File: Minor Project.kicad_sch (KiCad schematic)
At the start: 32 parts, among them J1 Conn_Coaxial, J2 Conn_Coaxial, J3 Conn_Coaxial, J4 Conn_Coaxial, J5 Conn_Coaxial, J6 Conn_Coaxial, J7 Conn_Coaxial, J8 Conn_Coaxial, J9 Conn_Coaxial, U1 HMC596LP4E, U2 HMC596LP4E, U3 HMC595A, U4 DPX165850DT-8085D3, U5 HMC8410LP2FE, U6 ADL5507ACBZ

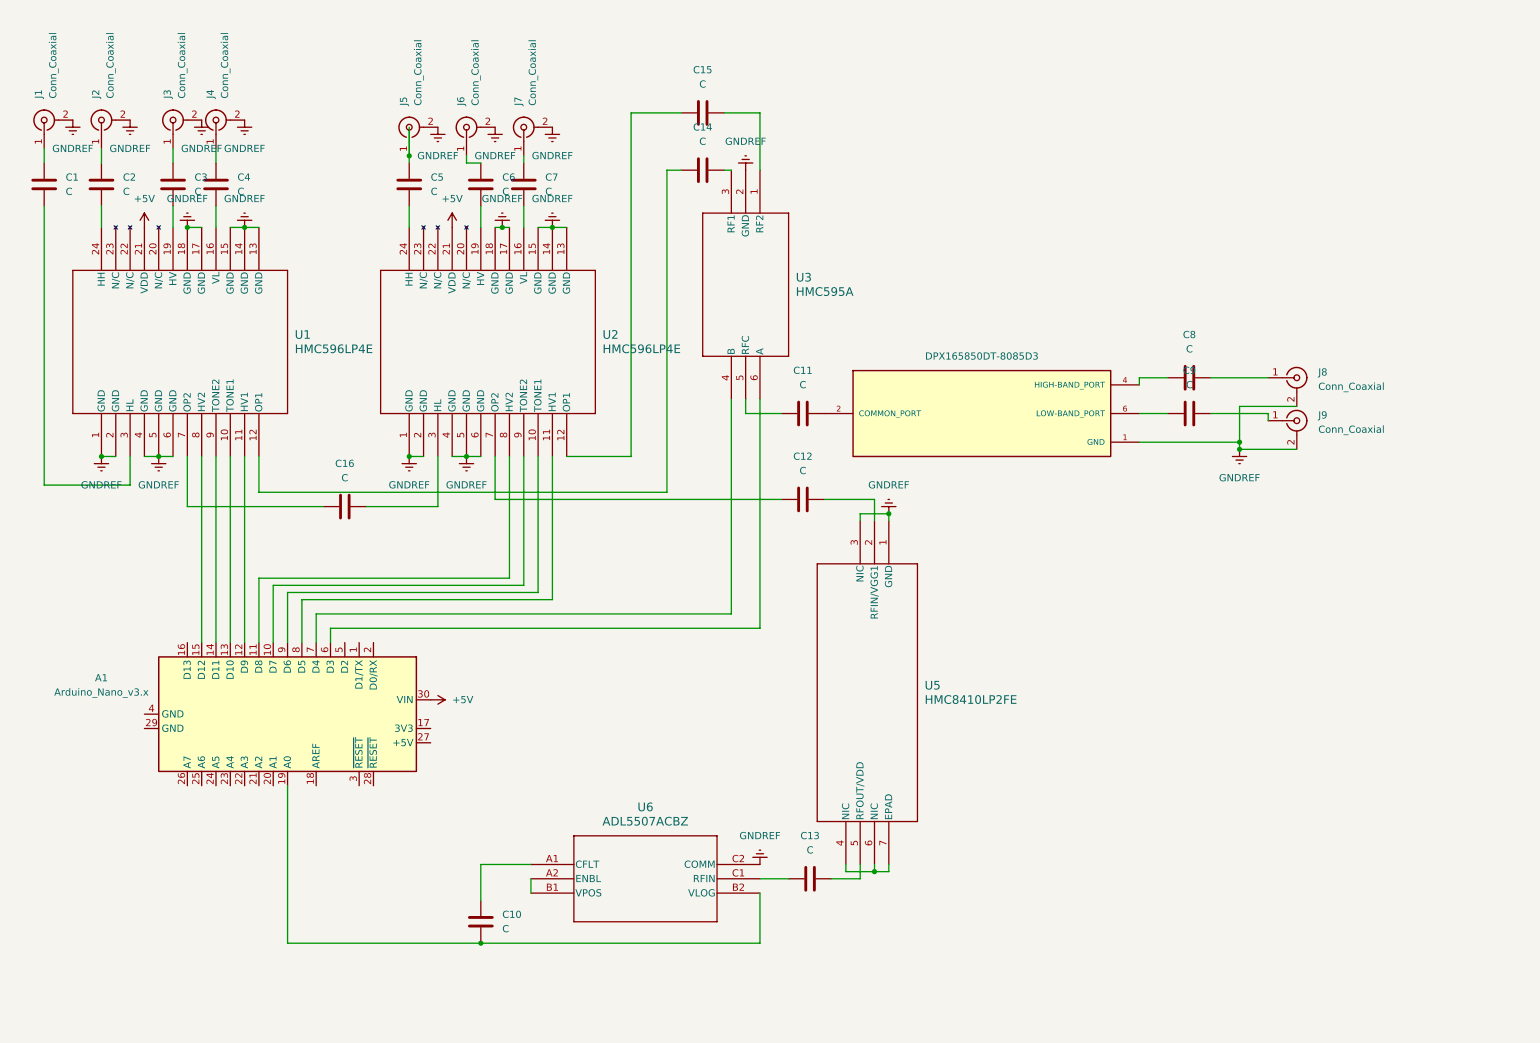
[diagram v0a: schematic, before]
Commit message: refactor schematic
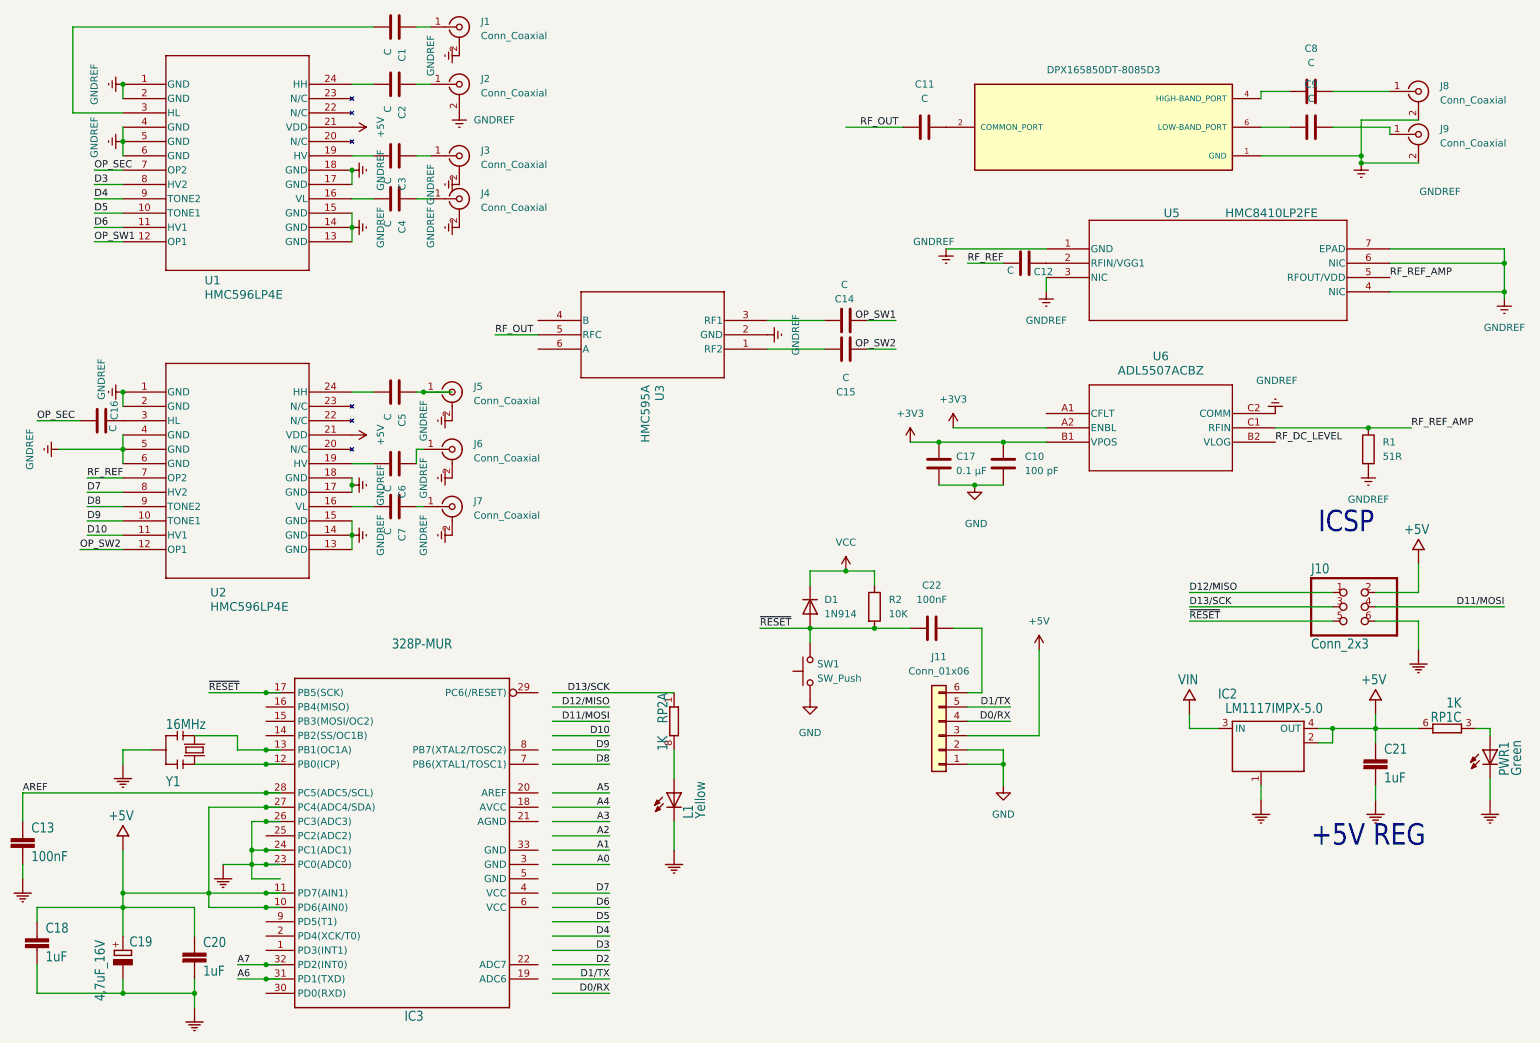
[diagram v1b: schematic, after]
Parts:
- removed A1: Arduino_Nano_v3.x, Module:Arduino_Nano, symbol MCU_Module:Arduino_Nano_v3.x
- removed C13: C, Capacitor_SMD:C_0402_1005Metric, symbol Device:C
- added C13: 100nF, NanoV3.3:C_0603_1608Metric, symbol NanoV3.3:C
- added C17: 0.1 μF, Capacitor_SMD:C_0805_2012Metric_Pad1.18x1.45mm_HandSolder, symbol Device:C
- added C18, C20, C21: 1uF, NanoV3.3:C_0603_1608Metric, symbol NanoV3.3:C
- added C19: 4,7uF_16V, NanoV3.3:CP_EIA-3216-18_Kemet-A, symbol NanoV3.3:C_Polarized
- added C22: 100nF, Capacitor_SMD:C_0805_2012Metric_Pad1.18x1.45mm_HandSolder, symbol Device:C
- added D1: 1N914, Diode_THT:D_DO-35_SOD27_P7.62mm_Horizontal, symbol Diode:1N914
- added IC2: LM1117IMPX-5.0, NanoV3.3:SOT-223, symbol NanoV3.3:LM1117
- added IC3: 328P-MUR, NanoV3.3:VQFN-32-1EP_5x5mm_P0.5mm_EP3.254x3.254mm, symbol NanoV3.3:ATmega328P-VQFN
- added J10: Conn_2x3, NanoV3.3:PinHeader_2x3_P2.54mm_Vertical, symbol NanoV3.3:Conn_2x3
- added J11: Conn_01x06, FTDI HEADER:FTDI_Header, symbol Connector_Generic:Conn_01x06
- added L1: Yellow, LED_SMD:LED_0805_2012Metric, symbol NanoV3.3:LED
- added PWR1: Green, LED_SMD:LED_0805_2012Metric, symbol NanoV3.3:LED
- added R1: 51R, Resistor_SMD:R_0805_2012Metric_Pad1.20x1.40mm_HandSolder, symbol Device:R
- added R2: 10K, Resistor_SMD:R_0805_2012Metric_Pad1.20x1.40mm_HandSolder, symbol Device:R
- added RP1, RP2: 1K, Resistor_SMD:R_0805_2012Metric_Pad1.20x1.40mm_HandSolder, symbol NanoV3.3:R_Pack4_Split
- added SW1: SW_Push, Button_Switch_SMD:SW_MEC_5GSH9, symbol Switch:SW_Push
- added Y1: 16MHz, NanoV3.3:Resonator_SMD_Murata_CSTxExxV-3Pin_3.0x1.1mm, symbol NanoV3.3:Resonator
- C10: value C -> 100 pF; footprint Capacitor_SMD:C_0402_1005Metric -> Capacitor_SMD:C_0805_2012Metric_Pad1.18x1.45mm_HandSolder
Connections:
- net +5V: now also C18.1, C19.1 (+), C20.1, C21.1, IC2.2, IC2.4 (OUT), IC3.10 (PD6(AIN0)), IC3.11 (PD7(AIN1)), IC3.27 (PC4(ADC4/SDA)), J10.2, J11.3 (Pin_3), RP1.6 (2)
- net GND: now also C10.2, U5.4 (NIC), U5.6 (NIC), U5.7 (EPAD), C17.2, J11.1 (Pin_1), J11.2 (Pin_2), R1.2, SW1.1
- net OP_SW2: now reaches C15.1, U2.12 (OP1)
- net D8: now reaches U2.9 (TONE2)
- net D7: now reaches U2.8 (HV2)
- net D6: now reaches U1.11 (HV1)
- net D5: now reaches U1.10 (TONE1)
- net D4: now reaches U1.9 (TONE2)
- net D3: now reaches U1.8 (HV2)
- net +3V3: now reaches C10.1
- net +3V3: now also U6.A2 (ENBL), U6.B1 (VPOS), C17.1; no longer U6.B2 (VLOG)
- net D10: now reaches U2.11 (HV1)
- net D9: now reaches U2.10 (TONE1)
- net RF_OUT: now reaches C11.1, U3.5 (RFC)
- net at U2.3 (HL): now also C16.1; no longer C16.2
- net at C12.1: now also U5.2 (RFIN/VGG1); no longer U2.7 (OP2)
- net OP_SEC: now reaches U1.7 (OP2)
- net OP_SEC: now also C16.2; no longer C16.1
- net OP_SW1: now reaches C14.1, U1.12 (OP1)
- net RF_REF: now reaches C12.2
- net RF_REF: now also U2.7 (OP2); no longer U5.2 (RFIN/VGG1)
- net RF_REF_AMP: now reaches U5.5 (RFOUT/VDD)
- net RF_REF_AMP: now also U6.C1 (RFIN), R1.1
- net at U6.A1 (CFLT): no longer C10.2
- new net: L1.1, RP2.8 (2)
- new net: C22.2, J11.6 (Pin_6)
- new net: PWR1.1, RP1.3 (1)
- new net: IC3.12 (PB0(ICP)), Y1.1
- new net: IC3.13 (PB1(OC1A)), Y1.3
- new net A6: IC3.31 (PD1(TXD))
- new net A7: IC3.32 (PD2(INT0))
- new net AREF: C13.1, IC3.28 (PC5(ADC5/SCL))
- new net COM: C13.2, C18.2, C19.2 (-), C20.2, C21.2, IC2.1 (GND/ADJ), IC3.23 (PC0(ADC0)), IC3.24 (PC1(ADC1)), IC3.26 (PC3(ADC3)), J10.6, L1.2, PWR1.2, Y1.2
- new net D0/RX: J11.4 (Pin_4)
- new net D11/MOSI: J10.4
- new net D12/MISO: J10.1
- new net D13/SCK: J10.3, RP2.1
- new net D1/TX: J11.5 (Pin_5)
- new net RF_DC_LEVEL: U6.B2 (VLOG)
- new net VCC: D1.1 (K), R2.1
- new net VIN: IC2.3 (IN)
- new net ~{RESET}: C22.1, D1.2 (A), IC3.17 (PB5(SCK)), J10.5, R2.2, SW1.2
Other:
- note added: "+5V REG"
- note added: "ICSP"
- moved on the sheet: C1, C11, C12, C14, C15, C16, C2, C3, C4, C5, C6, C7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
